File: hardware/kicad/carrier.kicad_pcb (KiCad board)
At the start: 2 copper layers, 105 x 95 mm, 116 parts, among them J1 MC-107DMS, J10 J_ADS_MAIN ADSBee J5, J11 J_ADS_GNSS ADSBee J4, J2 J_NTC 103AT-2, J3 J_BAT JST-PH 2mm, J4 J_THERM 60C NC, J5 J_GNSS GPS-18037 J5, J6 J_ESP_A support, J7 J_ESP_B power/UART, J8 J_ESP_C I2C, J9 J_ESP_D support, Q1 2N7002, Q2 2N7002, Q3 2N7002, Q4 2N7002, Q5 MMBT3904, SW1 POWER JS102011SAQN (2=common), SW2 MUTE JS102011SAQN (2=common), U1 TPS70933DBVR, U10 BMP581, U2 TUSB320LAIRWBR, U3 SN74LVC1G02DBVR, U4 BQ25606RGER, U5 TLV840CADL29DBVR 2.9V, U6 TPS61088RHLR, U7 TPS22975DSGR, U8 MAX17048G+T10, U9 SN74LVC1G17DBVR

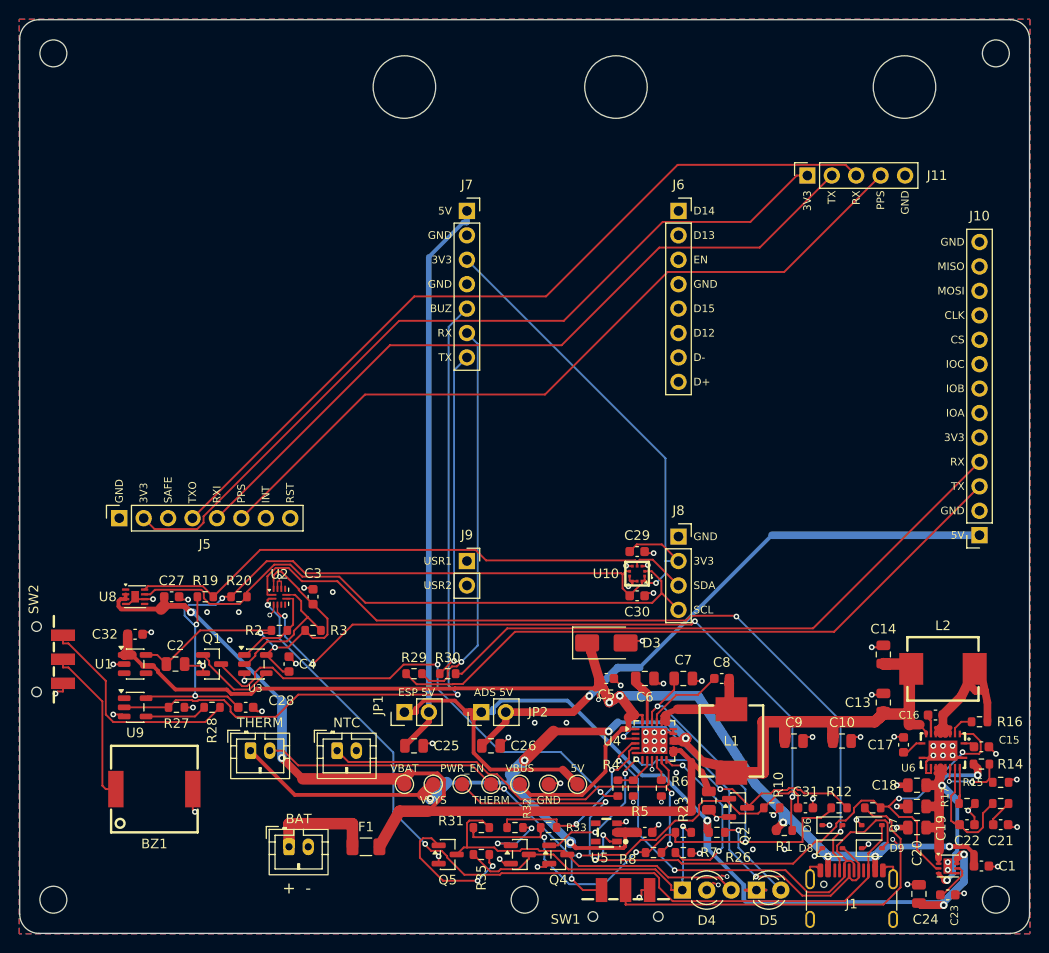
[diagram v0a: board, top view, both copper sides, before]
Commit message: Cleanups.
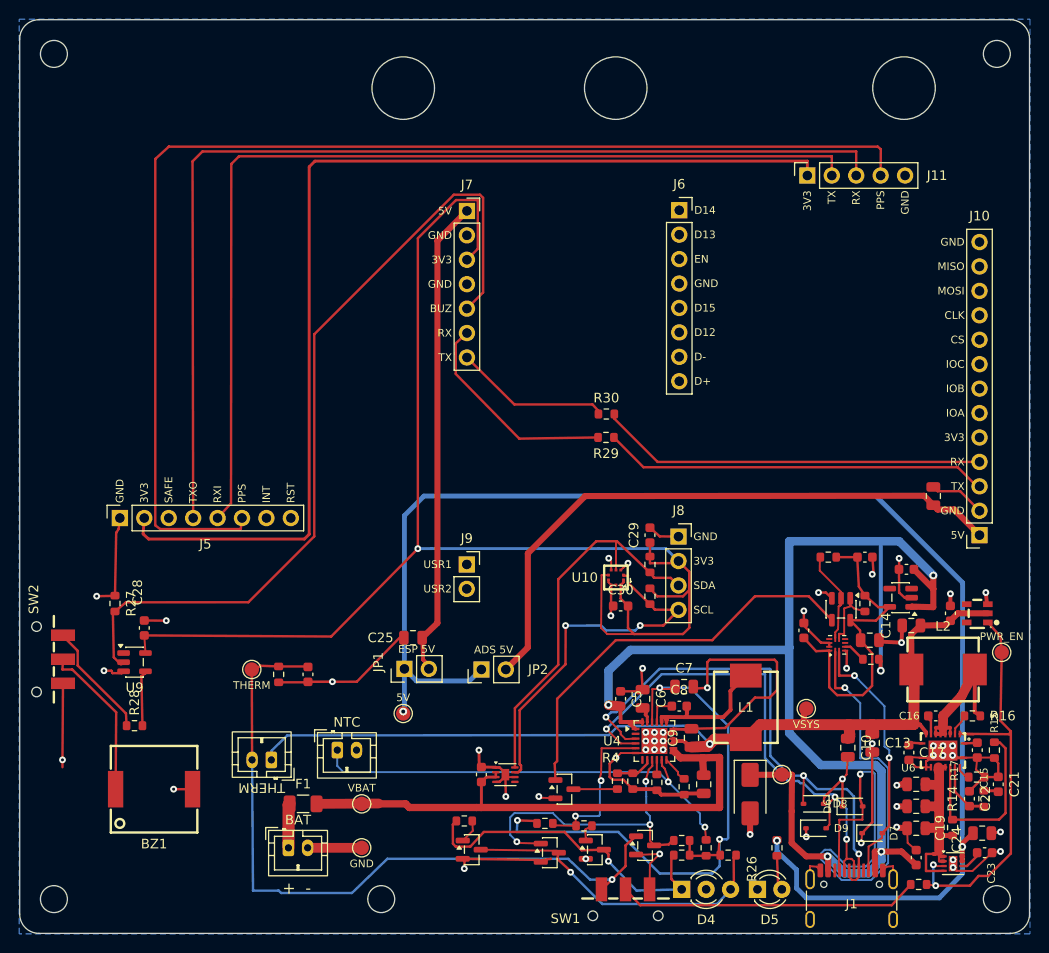
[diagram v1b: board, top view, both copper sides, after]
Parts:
- moved C32 80.5 mm to (92.2, 57.1), turned to 180 degrees
- moved U1 79.9 mm to (91.6, 60.1), turned to 180 degrees
- moved C2 72.2 mm to (88.4, 64.5)
- moved U3 61.2 mm to (85.4, 61.3), turned to -90 degrees
- moved R2 60.9 mm to (87.9, 60.7), turned to -90 degrees
- moved C4 60.9 mm to (87.9, 55.9), turned to 0 degrees
- moved U2 58.2 mm to (85.0, 65.0), turned to 90 degrees
- moved TP3 57.8 mm to (102.1, 65.8)
- moved R3 54.1 mm to (84.1, 55.9), turned to 180 degrees
- moved C31 53.6 mm to (30.0, 68.1), turned to -90 degrees
- moved R10 53.1 mm to (26.9, 68.1), turned to -90 degrees
- moved C26 52.8 mm to (95.0, 49.5), turned to 90 degrees
- moved C3 51.2 mm to (81.5, 63.5)
- moved R19 46.4 mm to (65.5, 56.6), turned to -90 degrees
- moved U5 44.8 mm to (99.6, 61.7)
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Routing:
- net GND: track 95.8 -> 229.1 mm, vias 89 -> 53
- net VBUS_DET: track 75.6 -> 2.39 mm, vias 4 -> 0
- net USB_CC2: track 89.2 -> 26.9 mm
- net RAIL_5V: track 97.5 -> 150.7 mm
- net ILIM_SW: track 51.6 -> 4.57 mm, vias 2 -> 0
- net GNSS_PPS: track 81.2 -> 127.0 mm
- net PWR_EN: track 86.9 -> 45.5 mm, vias 5 -> 2
- net VBAT: track 99.4 -> 61.3 mm, vias 2 -> 0
- net ILIM_HI: track 8.99 -> 42.6 mm
- net ADS_COMMS_TX: track 68.6 -> 40.1 mm
- net I2C_SCL: track 64.9 -> 38.3 mm, vias 0 -> 2
- net GNSS_3V3: track 85.1 -> 111.1 mm
- net GNSS_TXO: track 84.7 -> 109.0 mm
- net GNSS_RXI: track 78.7 -> 102.1 mm
- net ADS_COMMS_RX: track 63.6 -> 40.3 mm
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- removed copper zone on F.Cu, net GND
